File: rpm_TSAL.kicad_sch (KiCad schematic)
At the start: 2 parts, among them J1 Conn_01x02, J5 Conn_01x02

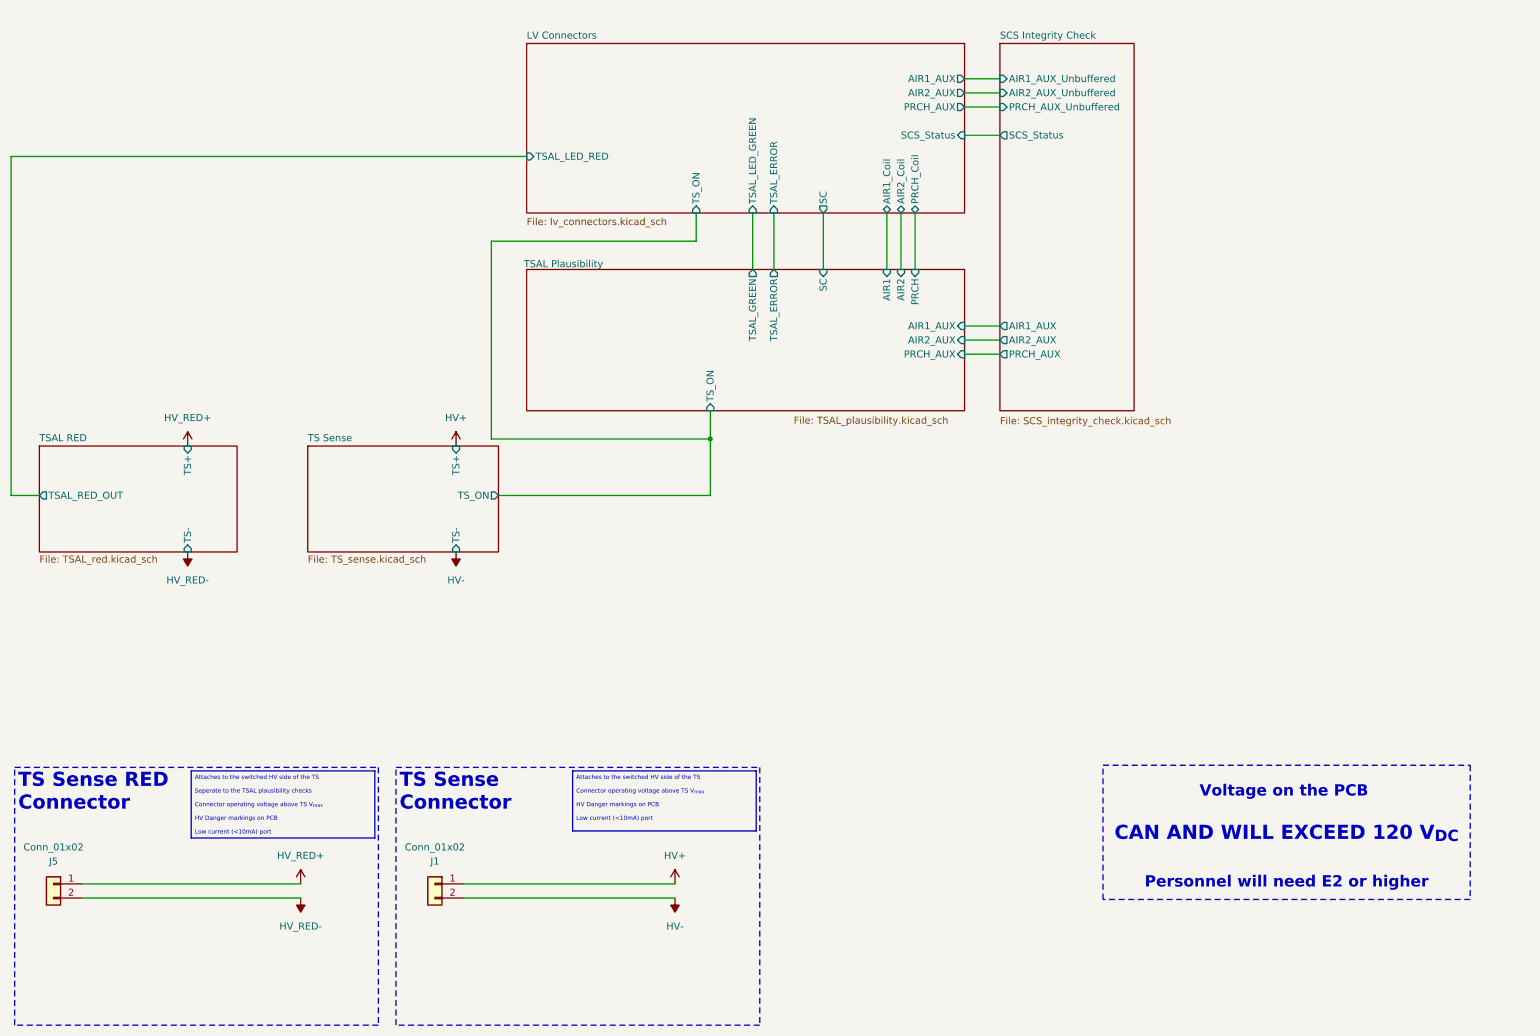
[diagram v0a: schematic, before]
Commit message: Added Rules
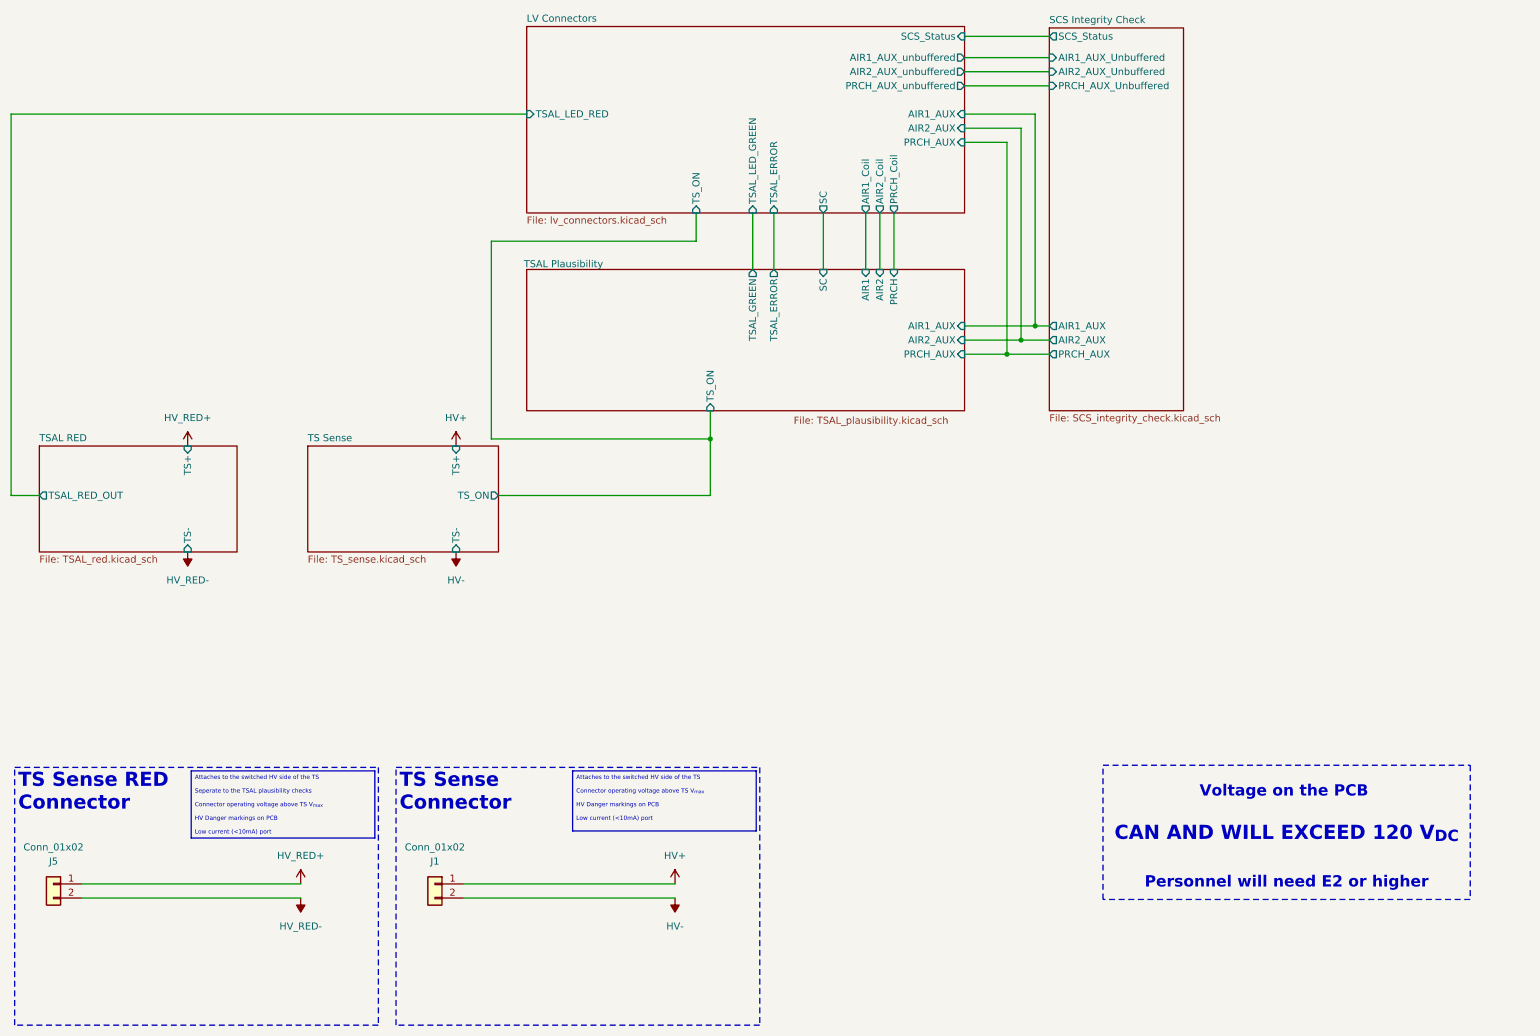
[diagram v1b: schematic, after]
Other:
- sheet LV Connectors ports: added AIR1_AUX_unbuffered, AIR2_AUX_unbuffered, PRCH_AUX_unbuffered; removed none
